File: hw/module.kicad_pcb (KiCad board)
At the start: 2 copper layers, 30 x 30 mm, 35 parts, among them Q1 MUN 2211, U1 CFPS-39, U2 CFPS-39, U3 74LVC1G125, U4 74 LVC 1G3157GW,125, U5 MAX919, U6 STM32L010F4P6, U7 BAS70-7-F, U8 SS39ET, U9 LM 61BIM3

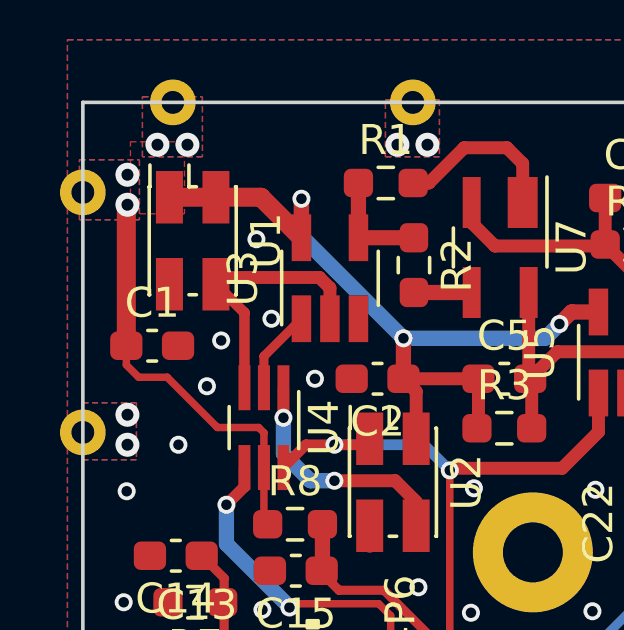
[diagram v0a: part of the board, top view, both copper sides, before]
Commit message: Add the last wire
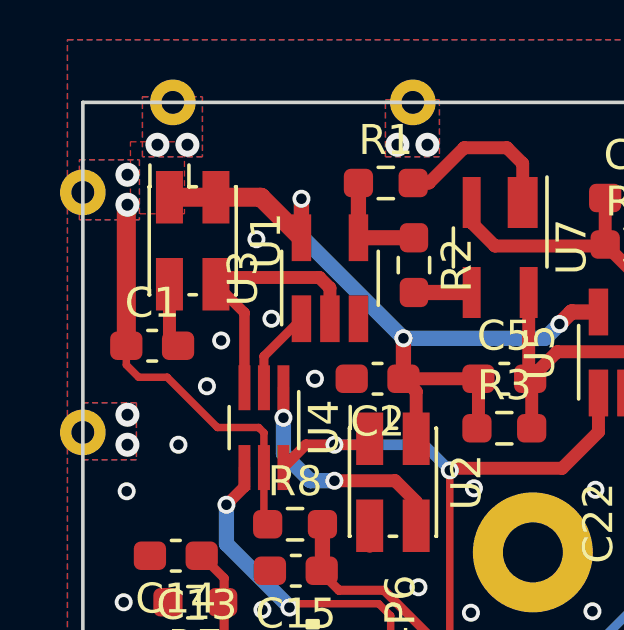
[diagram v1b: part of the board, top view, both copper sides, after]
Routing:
- net GND: track 3.34 -> 5.51 mm
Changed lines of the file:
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@@
   (segment (start 52.6 65) (end 55.224998 67.624998) (width 0.3048) (layer "B.Cu") (net 2))
   (segment (start 49.05 51.6) (end 49.05 50.55) (width 0.3048) (layer "F.Cu") (net 3))
+  (segment (start 45.9 48.15) (end 45.9 49.9125) (width 0.4318) (layer "F.Cu") (net 3))
   (segment (start 49.05 50.55) (end 50.3 49.3) (width 0.3048) (layer "F.Cu") (net 3))
   (segment (start 52.575 56.925) (end 52.575 56.4) (width 0.3556) (layer "F.Cu") (net 3))
+  (segment (start 45.9 49.9125) (end 46.1875 50.2) (width 0.4318) (layer "F.Cu") (net 3))
   (via (at 54.2 58.25) (size 0.6) (drill 0.35) (layers "F.Cu" "B.Cu") (free) (net 3))
   (via (at 54.525 64.65) (size 0.6) (drill 0.35) (layers "F.Cu" "B.Cu") (free) (net 3))
